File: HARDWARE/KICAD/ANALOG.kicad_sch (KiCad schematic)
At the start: 24 parts, among them J6 CONN 02x05 ODD EVEN, U6 LMV324, U7 ADS1115

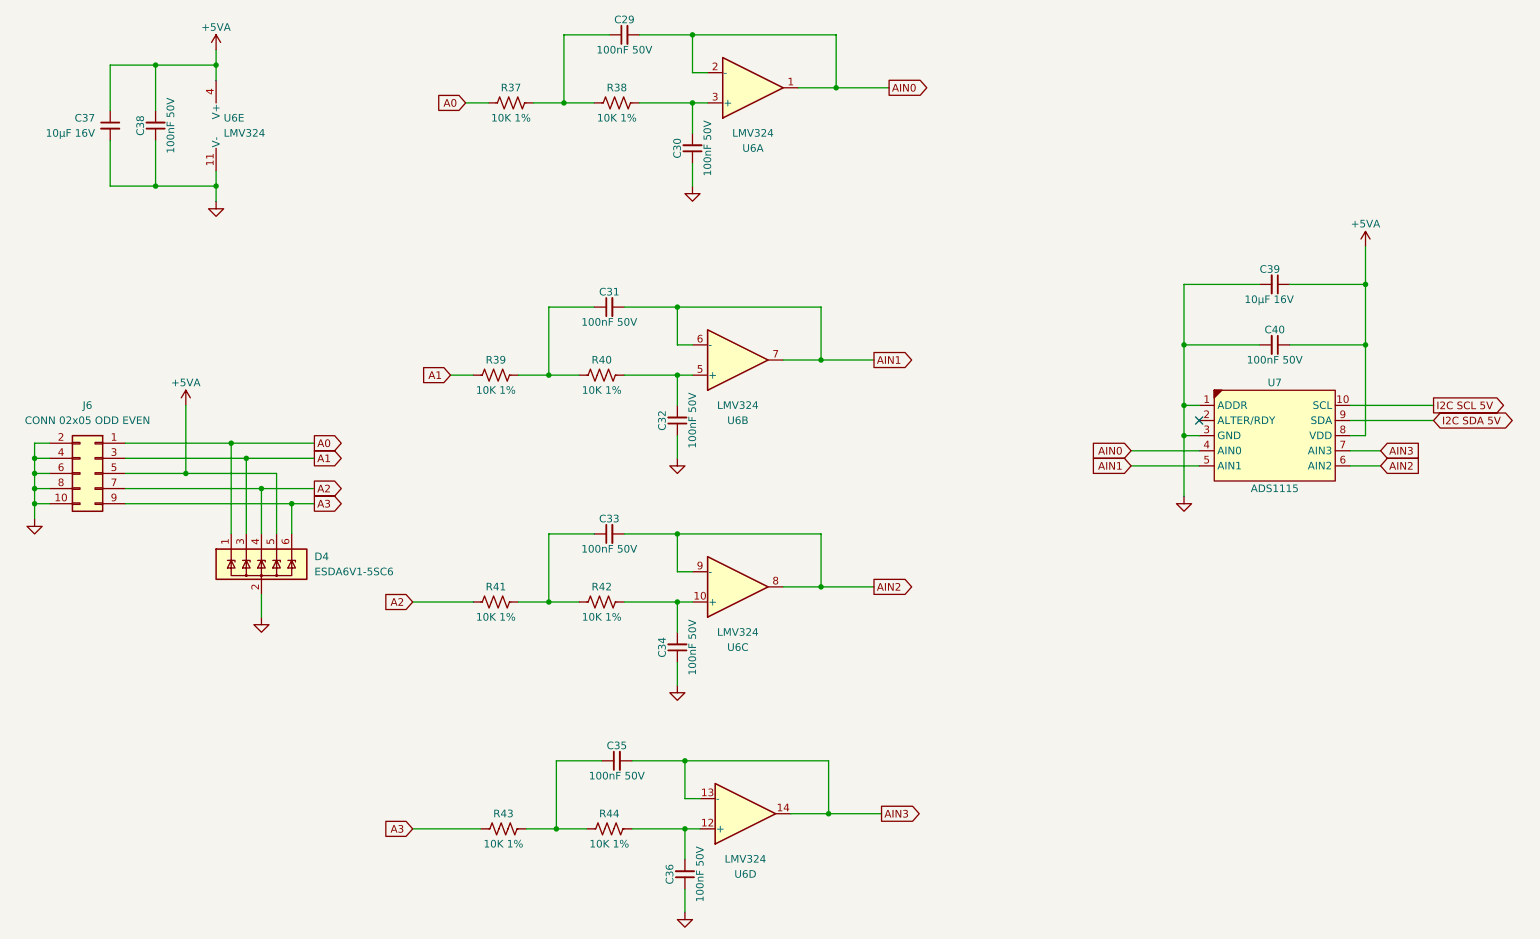
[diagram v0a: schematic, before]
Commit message: Refactoring.
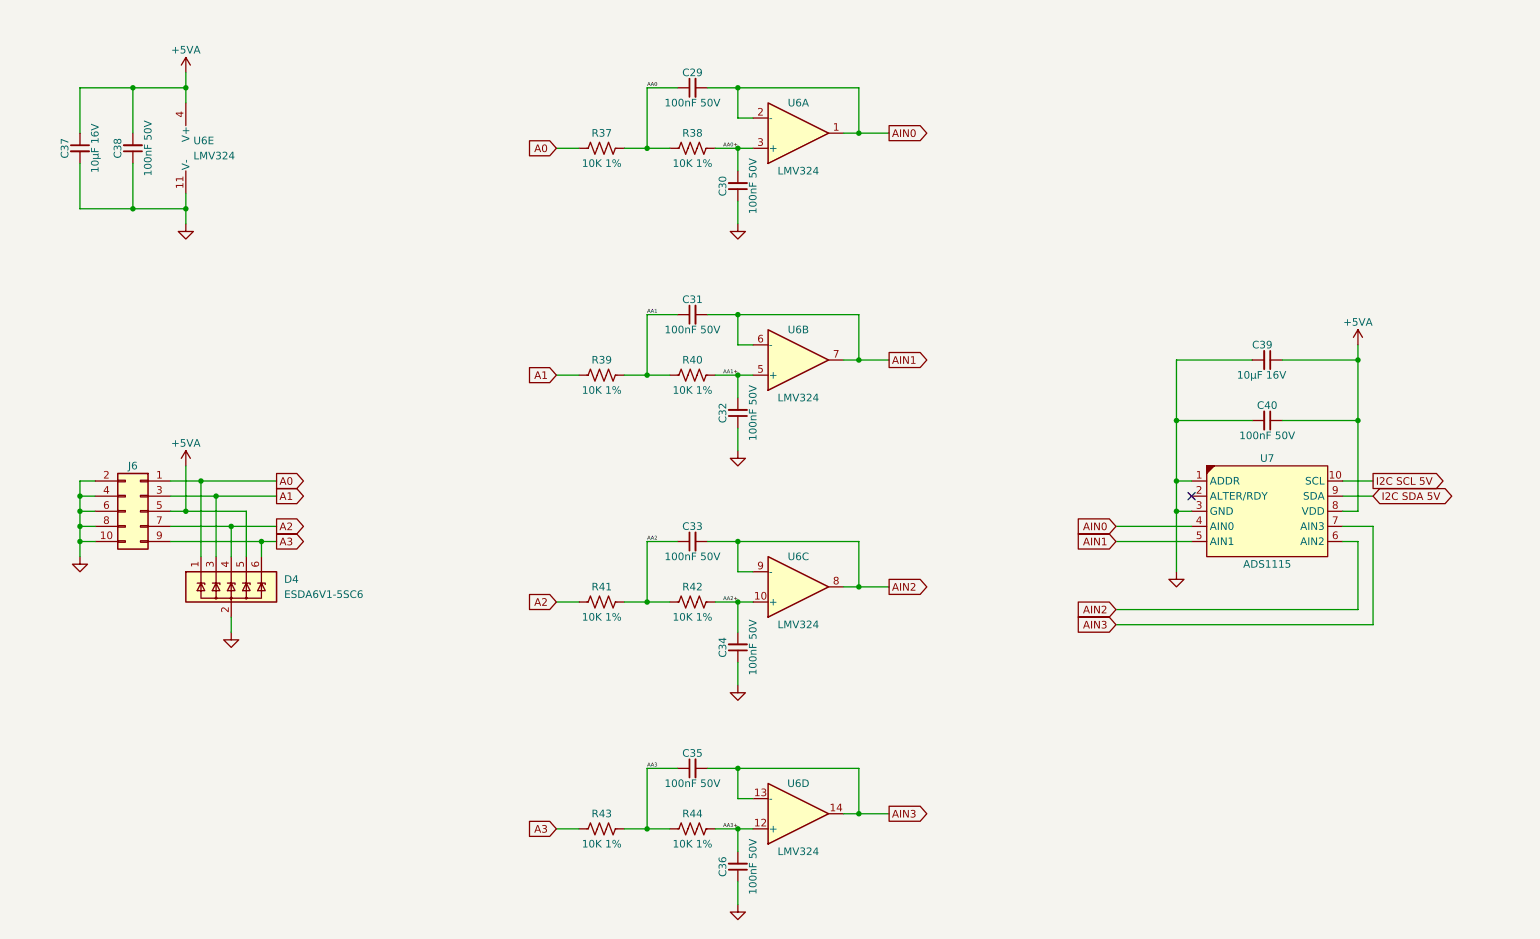
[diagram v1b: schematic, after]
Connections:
- net AA0: now reaches C29.1, R37.2, R38.1
- net AA0+: now reaches C30.2, R38.2, U6.3 (+)
- net AA2: now reaches C33.1, R41.2, R42.1
- net AA1+: now reaches C32.2, R40.2, U6.5 (+)
- net AA3: now reaches C35.1, R43.2, R44.1
- net AA3+: now reaches C36.2, R44.2, U6.12 (+)
- net AA2+: now reaches C34.2, R42.2, U6.10 (+)
- net AA1: now reaches C31.1, R39.2, R40.1
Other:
- moved on the sheet: C29, C30, C31, C32, C33, C34, C35, C36, C37, C38, C39, C40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
